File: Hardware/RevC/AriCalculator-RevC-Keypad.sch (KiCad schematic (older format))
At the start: 30 parts

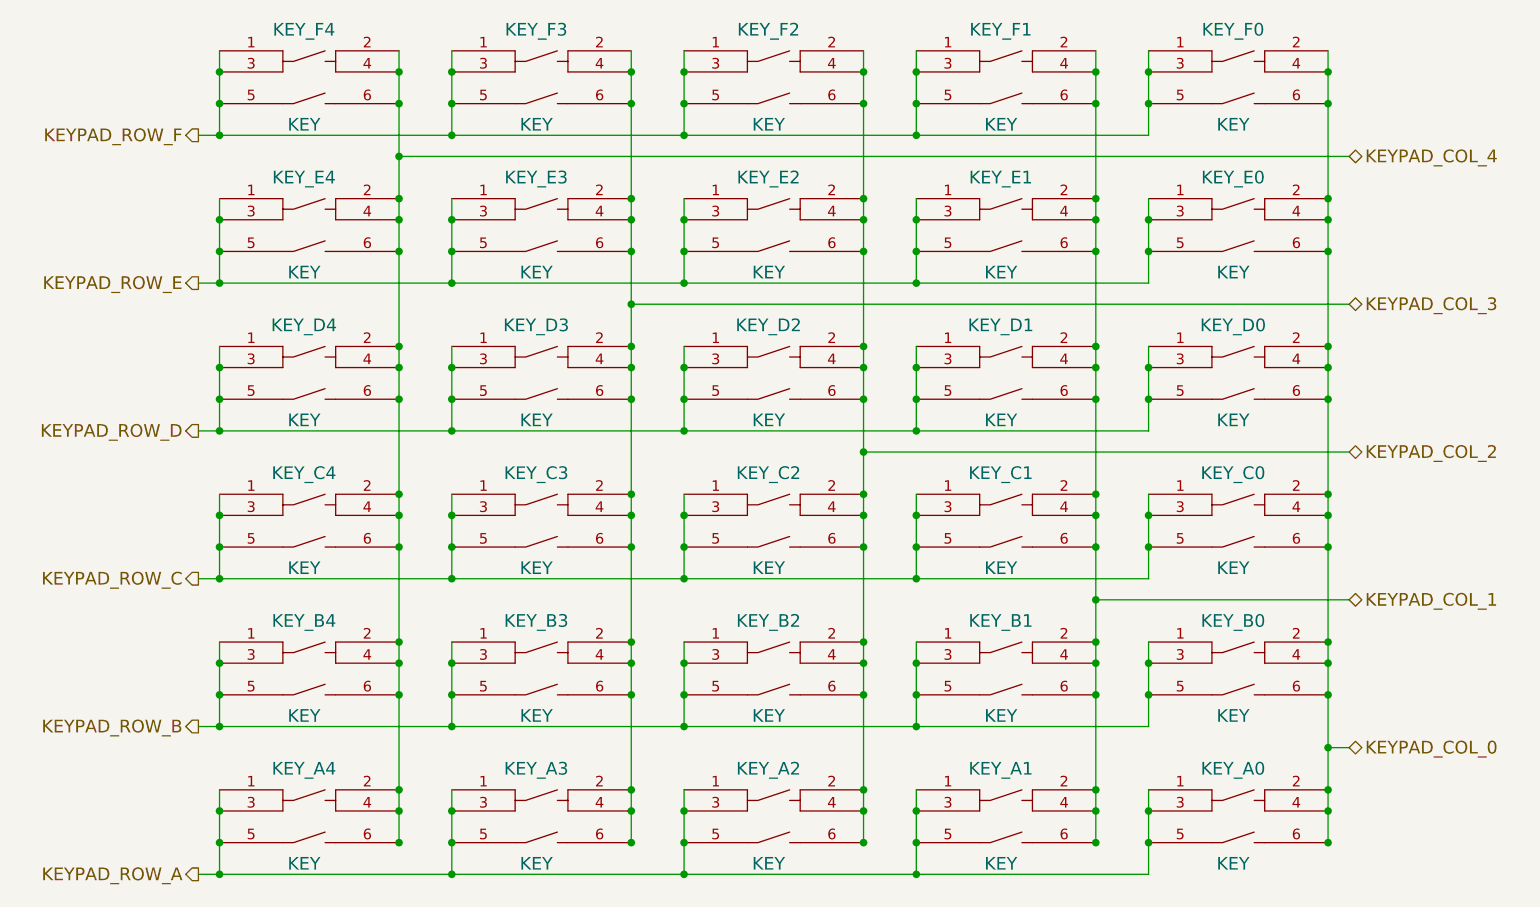
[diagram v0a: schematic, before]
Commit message: work in progress
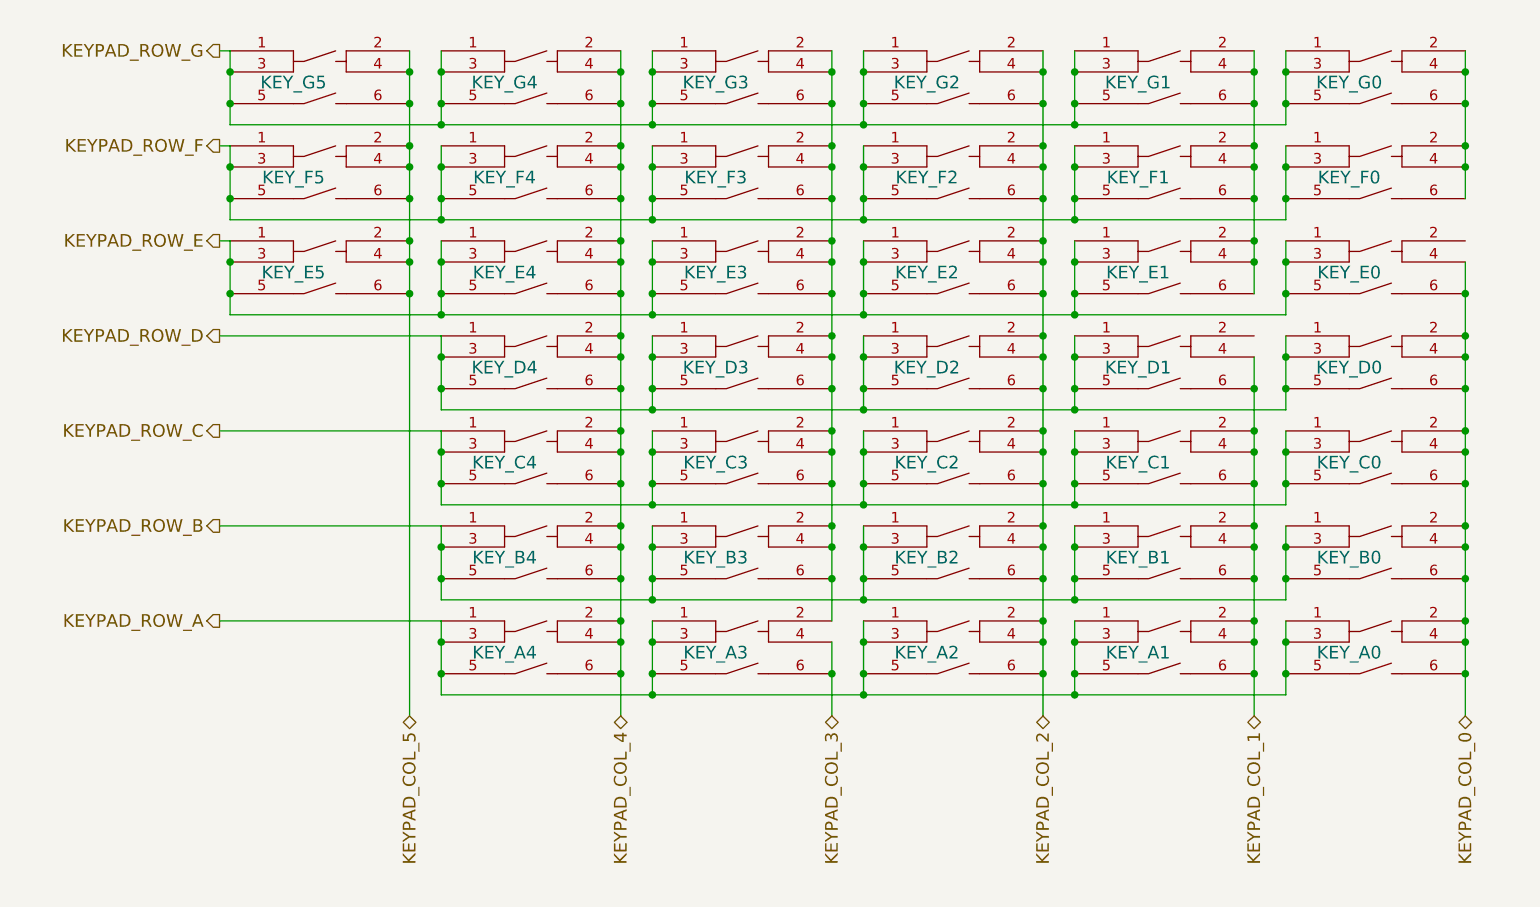
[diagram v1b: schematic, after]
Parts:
- added KEY_E5, KEY_F5, KEY_G0, KEY_G1, KEY_G2, KEY_G3, KEY_G4, KEY_G5: KEY, ~, symbol KEY
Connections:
- net KEYPAD_COL_0: no longer KEY_E0.2, KEY_F0.2, KEY_F0.4, KEY_F0.6
- net KEYPAD_COL_1: no longer KEY_D1.2, KEY_E1.2, KEY_E1.4, KEY_E1.6, KEY_F1.2, KEY_F1.4, KEY_F1.6
- net KEYPAD_COL_2: now also KEY_G2.2, KEY_G2.4, KEY_G2.6
- net KEYPAD_COL_3: no longer KEY_A3.2, KEY_B3.2, KEY_B3.4, KEY_B3.6, KEY_C3.2, KEY_C3.4, KEY_C3.6, KEY_D3.2, KEY_D3.4, KEY_D3.6, KEY_E3.2, KEY_E3.4, KEY_E3.6, KEY_F3.2, KEY_F3.4, KEY_F3.6
- net KEYPAD_COL_4: now also KEY_G4.2, KEY_G4.4, KEY_G4.6
- net KEYPAD_ROW_E: now also KEY_E5.1, KEY_E5.3, KEY_E5.5
- net KEYPAD_ROW_F: now also KEY_F5.1, KEY_F5.3, KEY_F5.5
- new net: KEY_A3.2, KEY_B3.2, KEY_B3.4, KEY_B3.6, KEY_C3.2, KEY_C3.4, KEY_C3.6, KEY_D3.2, KEY_D3.4, KEY_D3.6, KEY_E3.2, KEY_E3.4, KEY_E3.6, KEY_F3.2, KEY_F3.4, KEY_F3.6, KEY_G3.2, KEY_G3.4, KEY_G3.6
- new net: KEY_E1.2, KEY_E1.4, KEY_E1.6, KEY_F1.2, KEY_F1.4, KEY_F1.6, KEY_G1.2, KEY_G1.4, KEY_G1.6
- new net: KEY_F0.2, KEY_F0.4, KEY_F0.6, KEY_G0.2, KEY_G0.4, KEY_G0.6
- new net KEYPAD_COL_5: KEY_E5.2, KEY_E5.4, KEY_E5.6, KEY_F5.2, KEY_F5.4, KEY_F5.6, KEY_G5.2, KEY_G5.4, KEY_G5.6
- new net KEYPAD_ROW_G: KEY_G0.1, KEY_G0.3, KEY_G0.5, KEY_G1.1, KEY_G1.3, KEY_G1.5, KEY_G2.1, KEY_G2.3, KEY_G2.5, KEY_G3.1, KEY_G3.3, KEY_G3.5, KEY_G4.1, KEY_G4.3, KEY_G4.5, KEY_G5.1, KEY_G5.3, KEY_G5.5
